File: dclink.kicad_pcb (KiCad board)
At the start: 2 copper layers, 61.5 x 52.6 mm, 3 parts

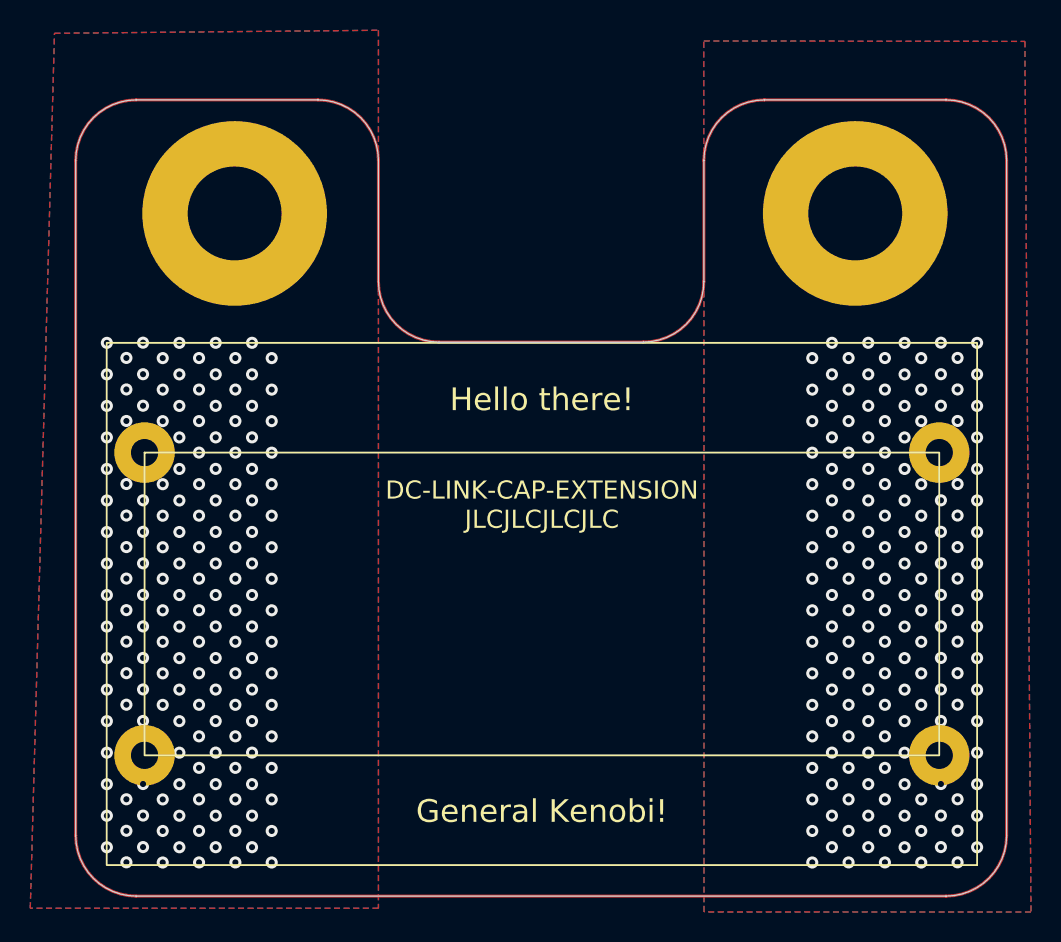
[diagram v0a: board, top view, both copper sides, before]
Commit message: add measurement
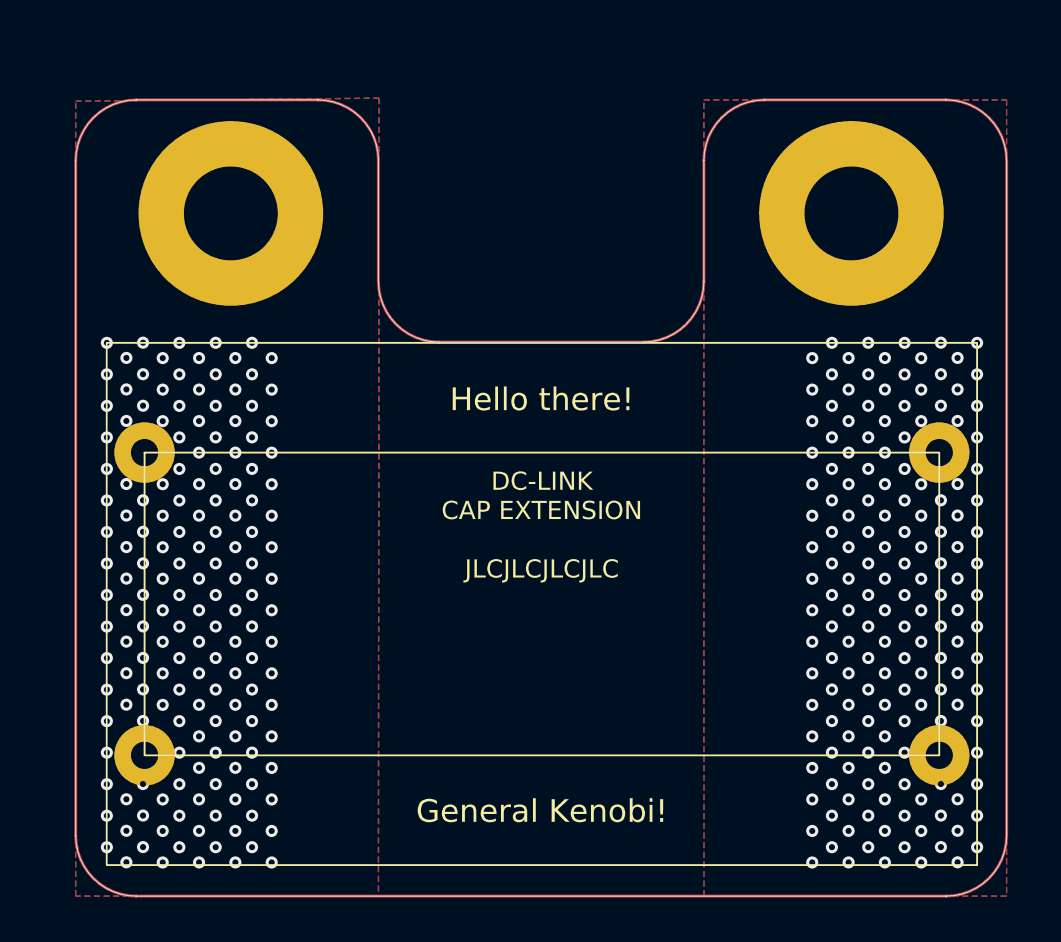
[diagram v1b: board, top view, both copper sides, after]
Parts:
- moved   0.25 mm to (170.3, 86.0)
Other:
- board text added: "DC-LINK CAP EXTENSION JLCJLCJLCJLC"
- board text removed: "CHECK:position of mounting holes: 86 or 86.5 in y: if the position of y is 86 there is the same distance between mounting hole and top bar and mounting hole and capacitor"
- board text removed: "DC-LINK-CAP-EXTENSION JLCJLCJLCJLC"

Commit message: minors
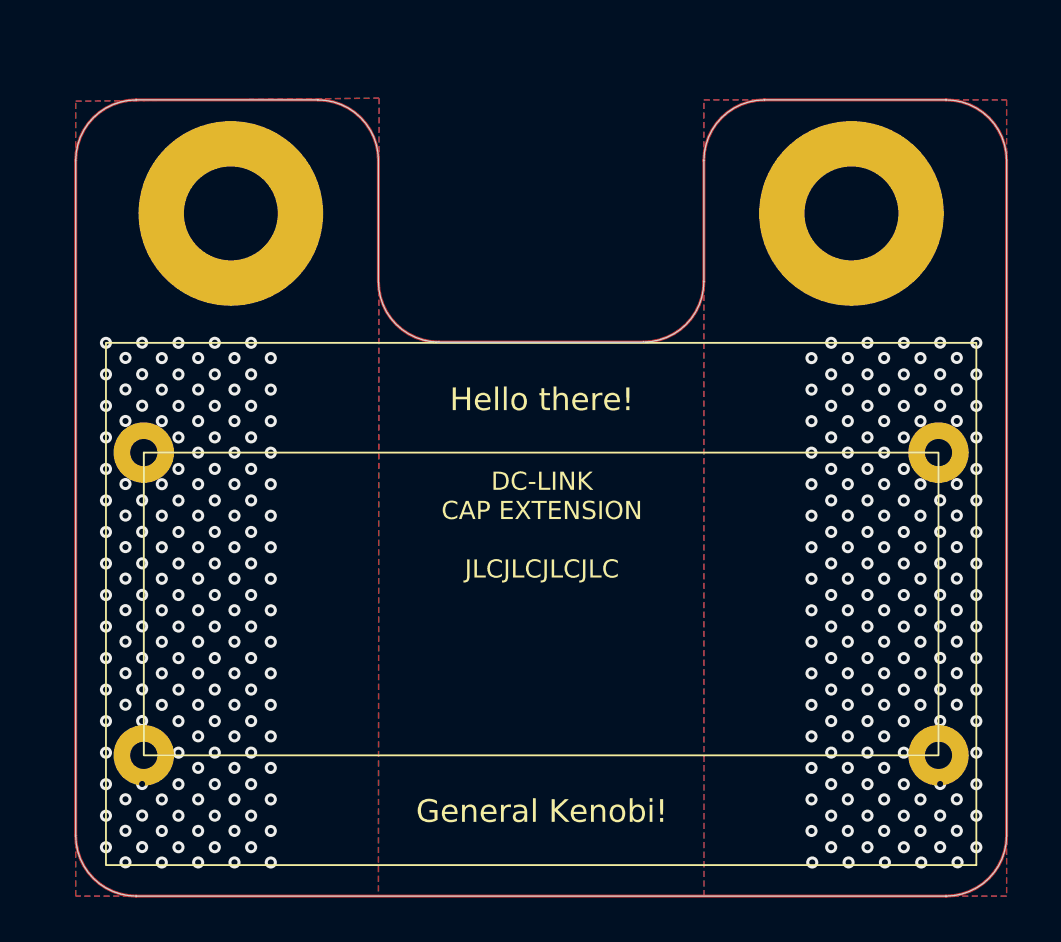
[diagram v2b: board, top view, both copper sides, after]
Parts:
- moved   0.05 mm to (149.8, 121.3)
